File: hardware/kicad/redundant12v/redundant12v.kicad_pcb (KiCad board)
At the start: 2 copper layers, 78 x 26.4 mm, 27 parts, among them J1 Conn_01x06, J2 IDC 2x5 Male, Q1 2N3904, Q2 2N3904, U1 ATtiny212-SS, U2 MAX232CPE, U3 LD1117S50TR_SOT223, X1 ASCO

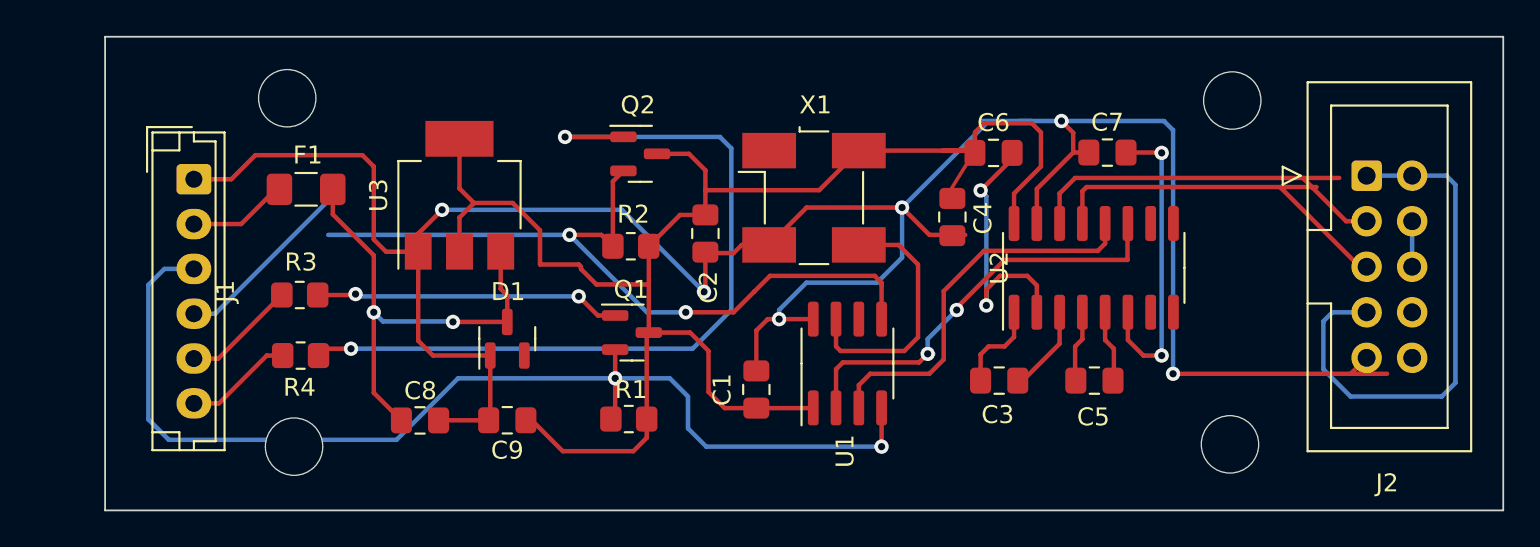
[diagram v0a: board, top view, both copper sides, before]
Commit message: PCB rev 1 finished
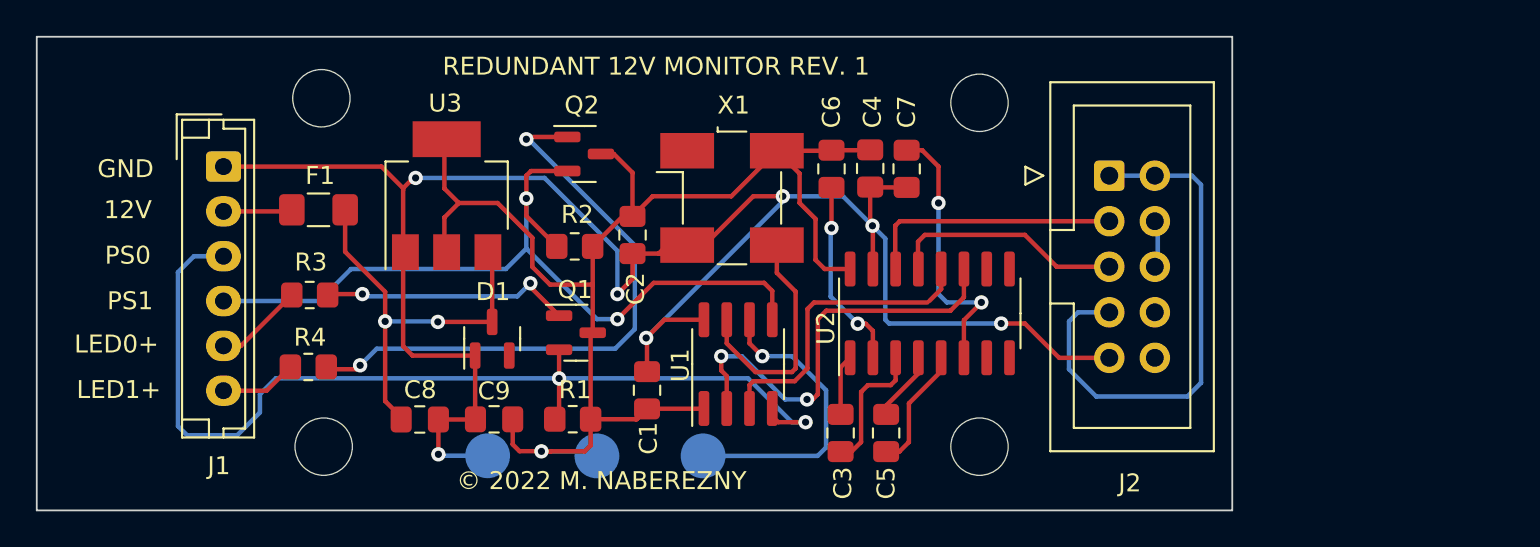
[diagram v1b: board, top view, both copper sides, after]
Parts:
- added TP1: GND, TestPoint:TestPoint_Pad_D2.5mm, B.Cu at (143.3, 103.6)
- added TP1: VTG_5V, TestPoint:TestPoint_Pad_D2.5mm, B.Cu at (149.4, 103.6)
- added TP2: UPDI, TestPoint:TestPoint_Pad_D2.5mm, B.Cu at (155.3, 103.6)
- moved J2 14.4 mm to (177.9, 88.0)
- moved REF** 14.1 mm to (170.7, 83.9)
- moved REF** 14.0 mm to (170.7, 103.1)
- moved C5 12.0 mm to (165.5, 102.4), turned to -90 degrees
- moved C7 11.2 mm to (166.6, 87.6), turned to 90 degrees
- moved U2 9.49 mm to (167.9, 95.7)
- moved C3 9.31 mm to (162.9, 102.4), turned to -90 degrees
- moved C6 9.08 mm to (162.4, 87.6), turned to -90 degrees
- moved C1 6.10 mm to (152.1, 100.0)
- moved U1 6.10 mm to (157.2, 98.5)
- moved C4 5.32 mm to (164.6, 87.6)
- moved X1 4.57 mm to (156.9, 89.3)
- moved C2 4.06 mm to (151.3, 91.3)
- moved Q2 3.13 mm to (148.6, 86.8)
- moved R2 3.13 mm to (148.1, 92.0)
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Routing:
- net GND: track 141.3 -> 111.7 mm, vias 6 -> 7
- net UPDI: track 0.00 -> 16.9 mm, vias 0 -> 1
- net Net-(Q2-Pad1): track 45.9 -> 33.7 mm
- net VCC: track 88.1 -> 77.3 mm, vias 0 -> 1
- net TX_12V: track 22.2 -> 14.5 mm
- net RX_12V: track 20.7 -> 13.1 mm
- net PS1: track 52.9 -> 45.9 mm
- net PS0: track 61.9 -> 55.9 mm
- net Net-(C6-Pad2): track 15.7 -> 10.6 mm
- net RX_5V: track 21.6 -> 17.1 mm
- net Net-(C8-Pad2): track 26.2 -> 23.0 mm
- net Net-(Q1-Pad1): track 17.1 -> 14.2 mm
- net Net-(C5-Pad2): track 4.03 -> 6.94 mm
- net Net-(C3-Pad2): track 4.94 -> 7.61 mm
- net Net-(C7-Pad2): track 17.1 -> 15.3 mm
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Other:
- board size 78 x 26.4 mm -> 66.7 x 26.4 mm
- board text added: "12V"
- board text added: "CTS"
- board text added: "DCD"
- board text added: "DSR"
- board text added: "DTR"
- board text added: "GND"
- board text added: "LED0+"
- board text added: "LED1+"
- board text added: "NC"
- board text added: "PS0"
- board text added: "PS1"
- board text added: "REDUNDANT 12V MONITOR REV. 1"
- board text added: "RI"
- board text added: "RTS"
- board text added: "RX"
- board text added: "TX"
- board text added: "UPDI"
- board text added: "VTG_5V"
- board text added: "© 2022 M. NABEREZNY"
